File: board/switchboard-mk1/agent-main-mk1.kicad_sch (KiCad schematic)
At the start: 17 parts, among them J1 Socket 02, J2 Socket 03, J3 Socket 01, J4 Socket 06, J5 Socket 05, J6 Socket 04, J7 Socket 07, J8 Socket 08, M1 Module_XIAO_Generic_SocketSMD

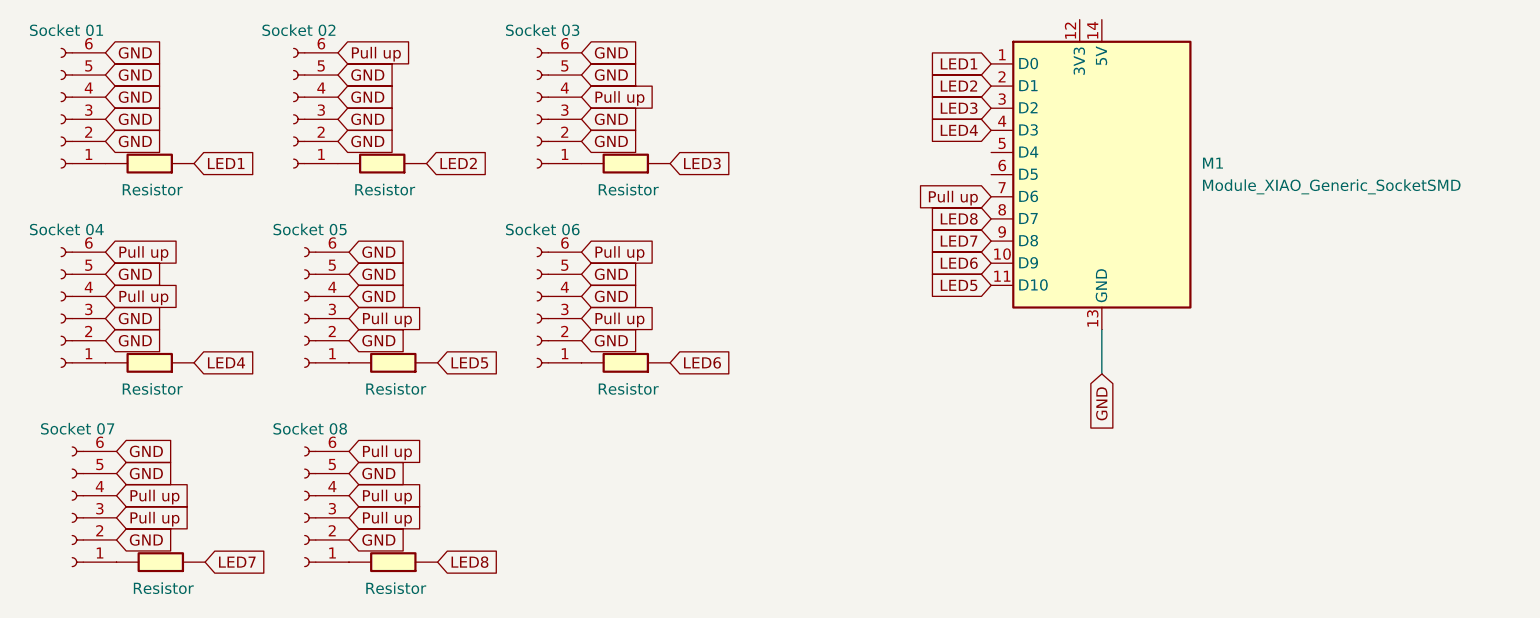
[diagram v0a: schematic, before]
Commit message: archive
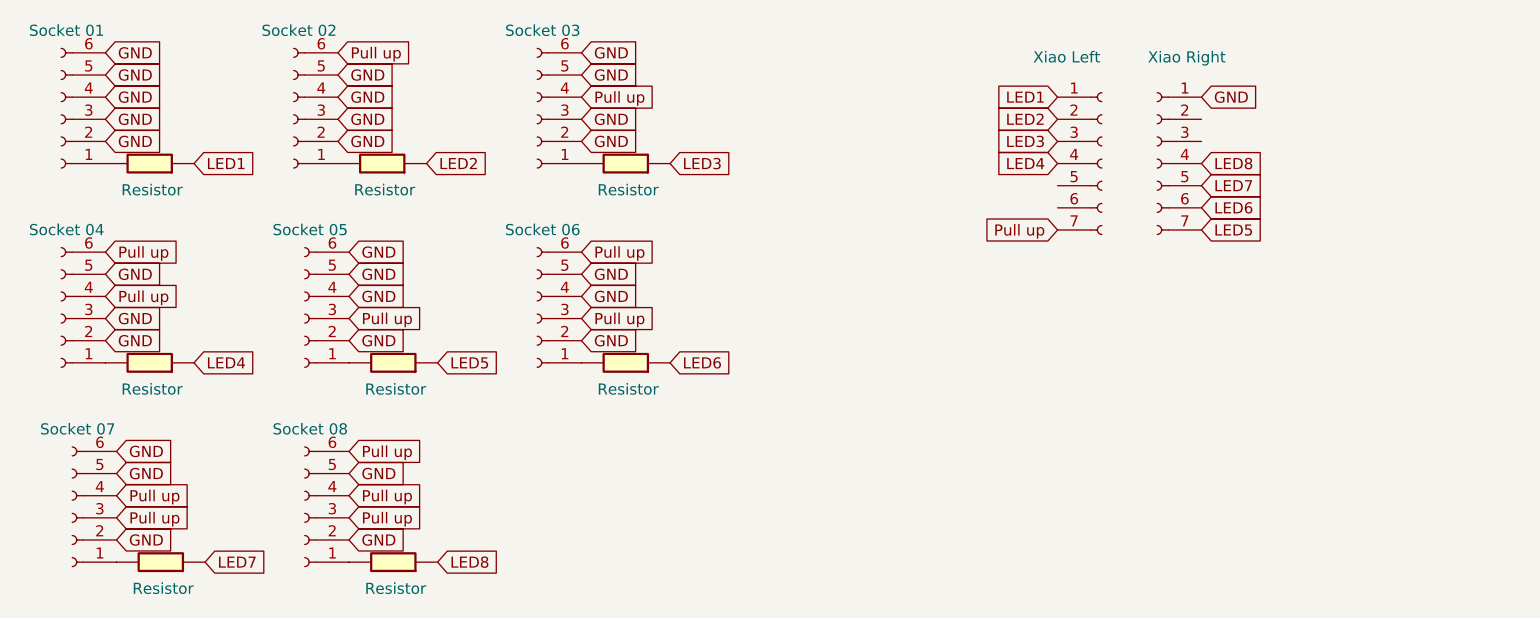
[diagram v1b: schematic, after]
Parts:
- removed M1: Module_XIAO_Generic_SocketSMD, fab:Module_XIAO_Generic_SocketSMD, symbol fab:Module_XIAO_Generic_SocketSMD
- added J10: Xiao Right, Connector_PinSocket_2.54mm:PinSocket_1x07_P2.54mm_Vertical, symbol Connector:Conn_01x07_Socket
- added J9: Xiao Left, Connector_PinSocket_2.54mm:PinSocket_1x07_P2.54mm_Vertical, symbol Connector:Conn_01x07_Socket
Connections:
- net GND: now also J10.1 (Pin_1)
- net LED1: now also J9.1 (Pin_1)
- net LED2: now also J9.2 (Pin_2)
- net LED3: now also J9.3 (Pin_3)
- net LED4: now also J9.4 (Pin_4)
- net LED5: now also J10.7 (Pin_7)
- net LED6: now also J10.6 (Pin_6)
- net LED7: now also J10.5 (Pin_5)
- net LED8: now also J10.4 (Pin_4)
- net Pull up: now also J9.7 (Pin_7)
